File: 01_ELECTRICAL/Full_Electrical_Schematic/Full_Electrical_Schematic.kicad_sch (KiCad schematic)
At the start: 17 parts, among them J1 Barrel_Jack, J10 Bullet_F, J11 Bullet_M, J12 Bullet_M, J13 Bullet_M, J14 Conn_01x03, J8 Bullet_F, J9 Bullet_F

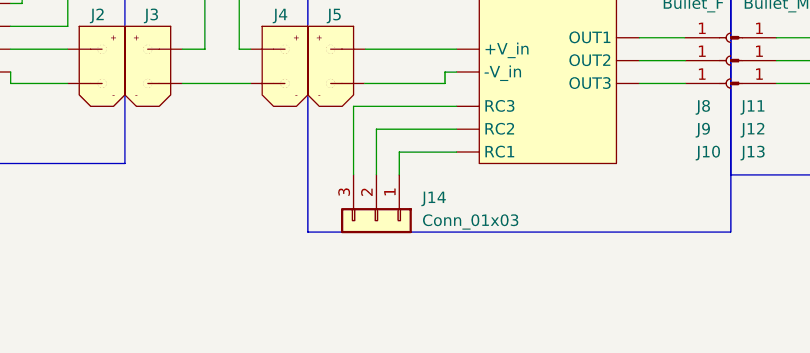
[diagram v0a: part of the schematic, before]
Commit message: Old kicad changes and BLDC CAD
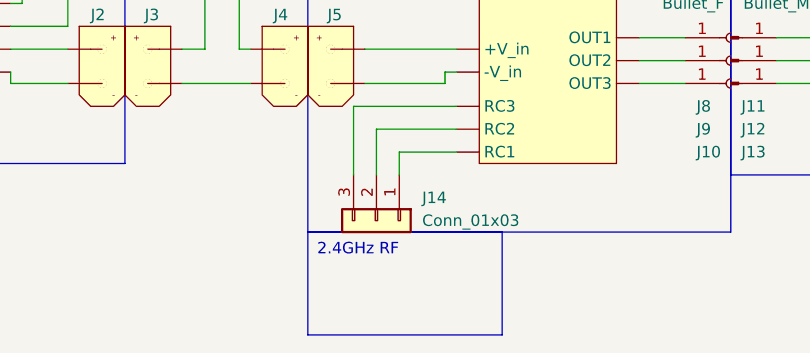
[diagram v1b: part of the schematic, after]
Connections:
- net at J3.: now also J4.; no longer J6.
- net at J4.: now also J6.; no longer J3.
- net at SC1. (RC3): now also J14.3 (Pin_3); no longer J5.
- net at B1. (GND): now also J1.2; no longer J2.
- net at M1. (SENS6): now also J11.1 (Pin_1)
- new net: J3., J6.
- new net: J5., SC1. (RC3)
- new net: B1. (GND), J2.
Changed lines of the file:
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@@
+		)
+	)
+	(text_box "2.4GHz RF"
+		(exclude_from_sim no)
+		(at 121.92 120.65 0)
+		(size 21.59 11.43)
+		(stroke
+			(width 0)
+			(type default)
+		)
+		(fill
+			(type color)
+			(color 255 49 217 0.3)
+		)
+		(effects
+			(font
+				(size 1.27 1.27)
+			)
+			(justify left top)
 		)
 	)
